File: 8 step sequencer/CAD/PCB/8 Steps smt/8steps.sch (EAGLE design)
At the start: 30 parts, among them IC1 4040N, IC2 4040N, IC3 7805TV, IC4 4051N, IC5 4051N, IC6 LM324N

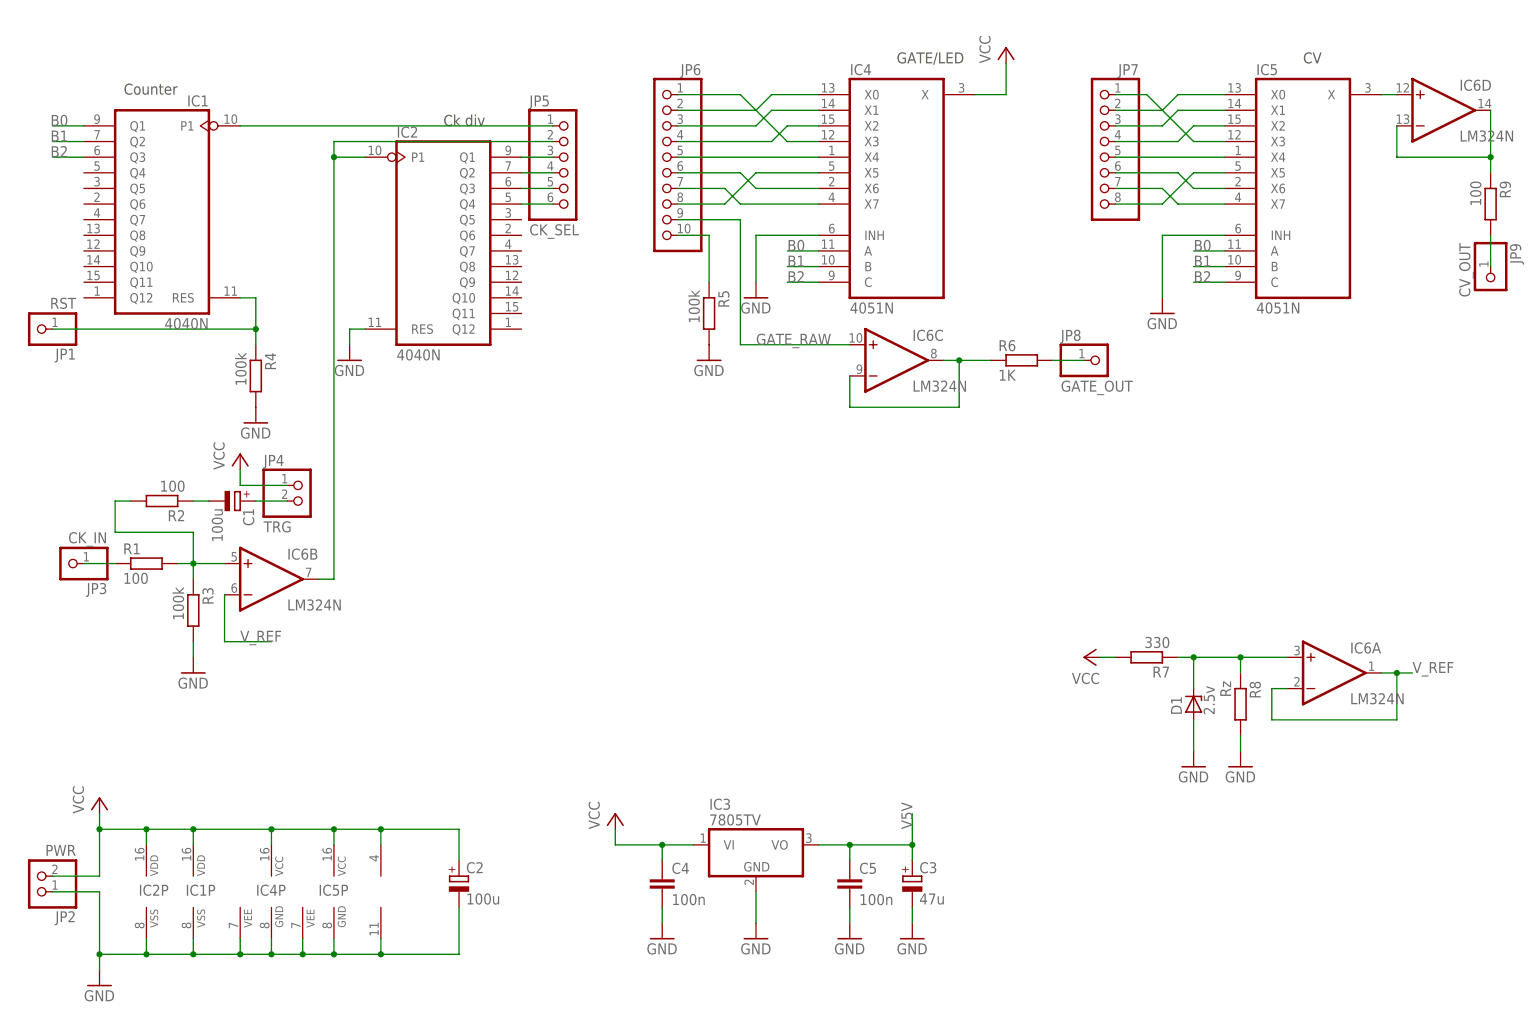
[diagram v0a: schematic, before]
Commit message: new fabrication files of  8 steps
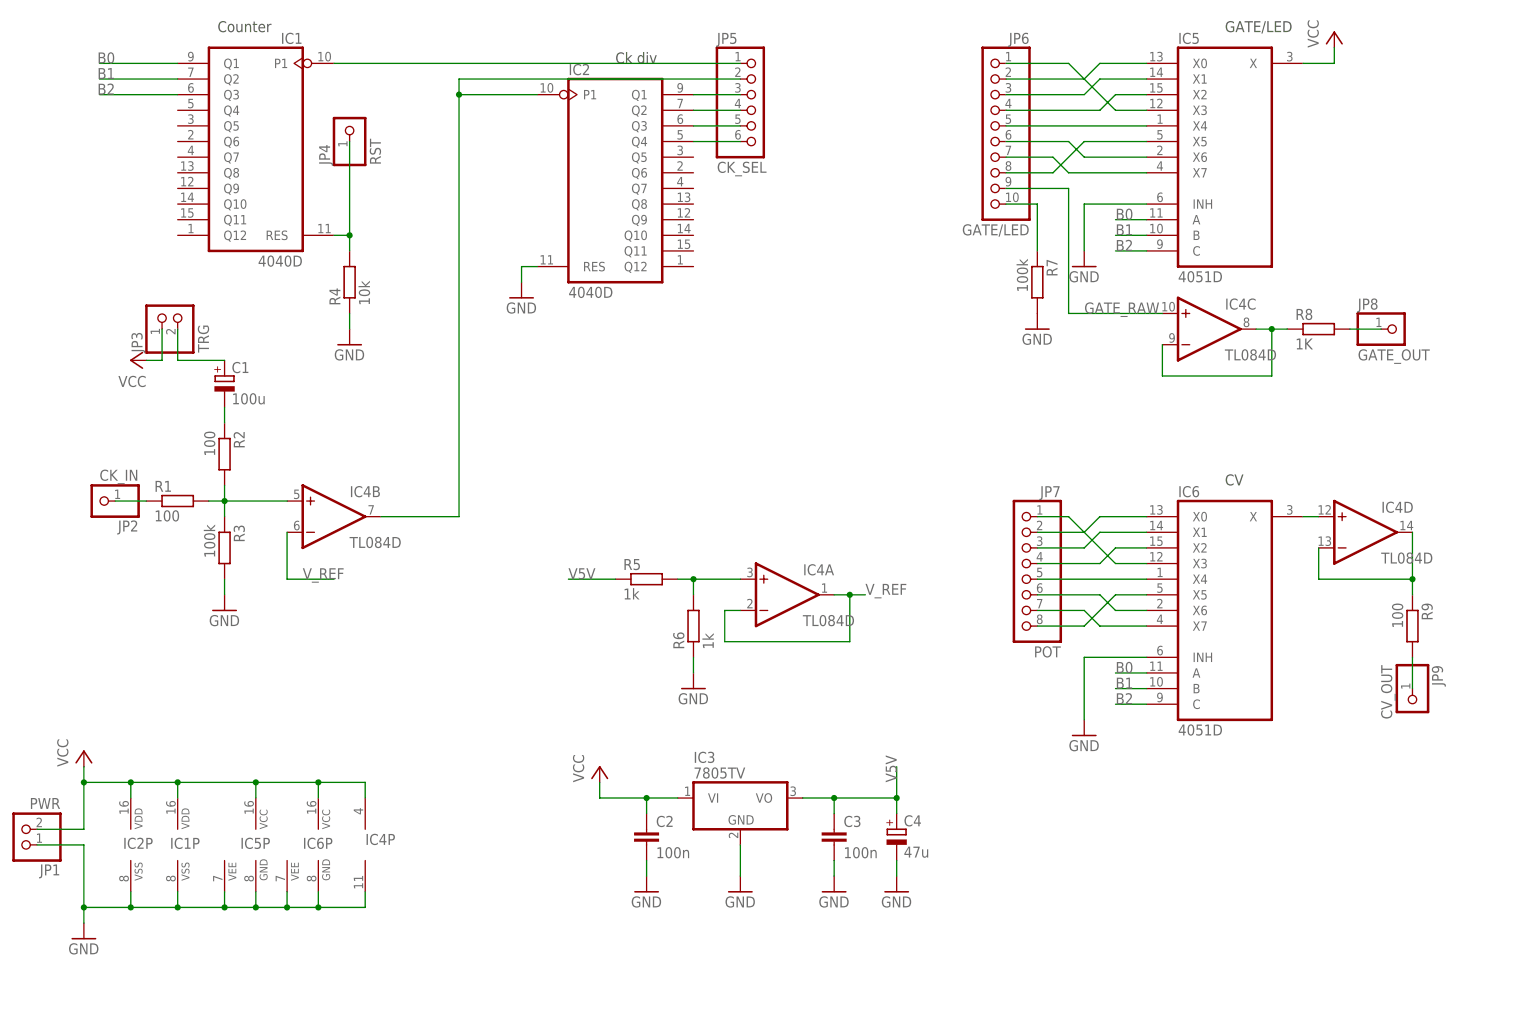
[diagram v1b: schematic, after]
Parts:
- removed C5: 100n, rcl:C-EU050-025X075
- removed D1: 2.5v, diode:ZENER-DIODEZD-2.5
- C1: device rcl:CPOL-EUE5-10.5 -> rcl:CPOL-EUE2.5-7
- C2: value 100u -> 100n; device rcl:CPOL-EUE5-10.5 -> rcl:C-EU050-025X075
- C3: value 47u -> 100n; device rcl:CPOL-EUE5-10.5 -> rcl:C-EU050-025X075
- C4: value 100n -> 47u; device rcl:C-EU050-025X075 -> rcl:CPOL-EUE2.5-7
- IC1, IC2: value 4040N -> 4040D; device 40xx:4040N -> 40xx:4040D
- IC4: value 4051N -> TL084D; device 40xx:4051N -> linear:TL084D
- IC5: value 4051N -> 4051D; device 40xx:4051N -> 40xx:4051D
- IC6: value LM324N -> 4051D; device linear:LM324N -> 40xx:4051D
- JP1: value RST -> PWR; device pinhead:PINHD-1X1 -> pinhead:PINHD-1X2
- JP2: value PWR -> CK_IN; device pinhead:PINHD-1X2 -> pinhead:PINHD-1X1
- JP3: value CK_IN -> TRG; device pinhead:PINHD-1X1 -> pinhead:PINHD-1X2
- JP4: value TRG -> RST; device pinhead:PINHD-1X2 -> pinhead:PINHD-1X1
- JP6: value (none) -> GATE/LED
- JP7: value (none) -> POT
- R1, R2, R3, R9: device rcl:R-EU_0207/2V -> rcl:R-EU_R0805
- R4: value 100k -> 10k; device rcl:R-EU_0207/2V -> rcl:R-EU_R0805
- R5: value 100k -> 1k; device rcl:R-EU_0207/2V -> rcl:R-EU_R0805
- R6: value 1K -> 1k; device rcl:R-EU_0207/2V -> rcl:R-EU_R0805
- R7: value 330 -> 100k; device rcl:R-EU_0207/2V -> rcl:R-EU_R0805
- R8: value Rz -> 1K; device rcl:R-EU_0207/2V -> rcl:R-EU_R0805
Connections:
- net B0: now also IC6A.A; no longer IC4A.A
- net B1: now also IC6A.B; no longer IC4A.B
- net B2: now also IC6A.C; no longer IC4A.C
- net GATE_RAW: now also IC4C.+IN; no longer IC6C.+IN
- net GND: now also C2.2, C3.2, C4.-, IC4P.V-, IC6A.INH, IC6P.GND, IC6P.VEE, JP1.1, R4.1, R6.1, R7.2; no longer C2.-, C3.-, C4.2, C5.2, D1.A, IC4A.INH, IC4P.GND, IC4P.VEE, IC6P.V-, JP2.1, R4.2, R5.2, R8.2
- net N$1: now also IC4A.+IN, R5.2, R6.2; no longer D1.C, IC6A.+IN, R7.1, R8.1
- net N$10: now also IC5A.X3; no longer IC4A.X3
- net N$11: now also IC5A.X0; no longer IC4A.X0
- net N$12: now also IC5A.X1; no longer IC4A.X1
- net N$13: now also IC5A.X2; no longer IC4A.X2
- net N$14: now also IC5A.X4; no longer IC4A.X4
- net N$15: now also IC5A.X7; no longer IC4A.X7
- net N$16: now also IC5A.X6; no longer IC4A.X6
- net N$17: now also IC5A.X5; no longer IC4A.X5
- net N$18: now also IC6A.X3; no longer IC5A.X3
- net N$19: now also IC6A.X0; no longer IC5A.X0
- net N$20: now also IC6A.X1; no longer IC5A.X1
- net N$21: now also IC6A.X2; no longer IC5A.X2
- net N$22: now also IC6A.X4; no longer IC5A.X4
- net N$23: now also IC6A.X7; no longer IC5A.X7
- net N$25: now also IC6A.X5; no longer IC5A.X5
- net N$26: now also IC4D.-IN, IC4D.OUT; no longer IC6D.-IN, IC6D.OUT
- net N$28: now also R7.1; no longer R5.1
- net N$29: now also JP4.1, R4.2; no longer JP1.1, R4.1
- net N$3: now also IC4D.+IN, IC6A.X; no longer IC5A.X, IC6D.+IN
- net N$30: now also IC4C.-IN, IC4C.OUT, R8.1; no longer IC6C.-IN, IC6C.OUT, R6.1
- net N$31: now also R8.2; no longer R6.2
- net N$32: now also IC6A.X6; no longer IC5A.X6
- net N$33: now also IC4B.+IN; no longer IC6B.+IN
- net N$34: now also JP3.2; no longer JP4.2
- net N$35: now also JP2.1; no longer JP3.1
- net N$4: now also IC4B.OUT; no longer IC6B.OUT
- net V5V: now also C3.1, C4.+, R5.1; no longer C3.+, C5.1
- net VCC: now also C2.1, IC4P.V+, IC5A.X, IC6P.VCC, JP1.2, JP3.1; no longer C2.+, C4.1, IC4A.X, IC4P.VCC, IC6P.V+, JP2.2, JP4.1, R7.2
- net V_REF: now also IC4A.-IN, IC4A.OUT, IC4B.-IN; no longer IC6A.-IN, IC6A.OUT, IC6B.-IN
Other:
- moved on the sheet: C1, IC1, IC1P, IC2, IC2P, IC3, IC5, IC5P, JP5, JP6, JP7, JP8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
